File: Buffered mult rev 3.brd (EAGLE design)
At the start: 100.3 x 17.1 mm, 28 parts, among them IC1 OPA4171, IC2 OPA2171, J1 EURO_POWER_HEADERFAT_PADS

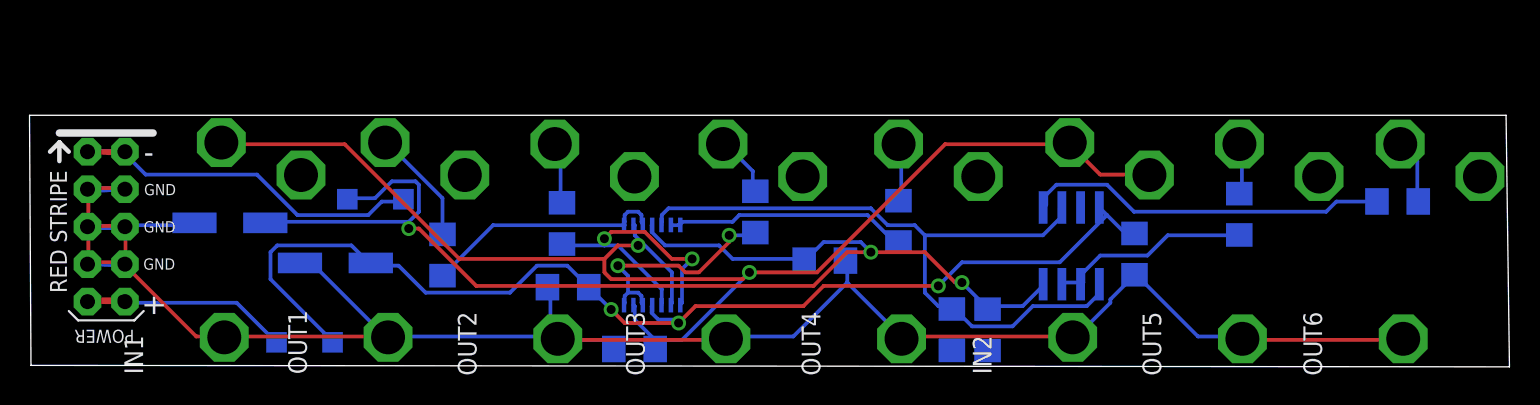
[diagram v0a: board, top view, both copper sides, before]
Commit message: minor changes
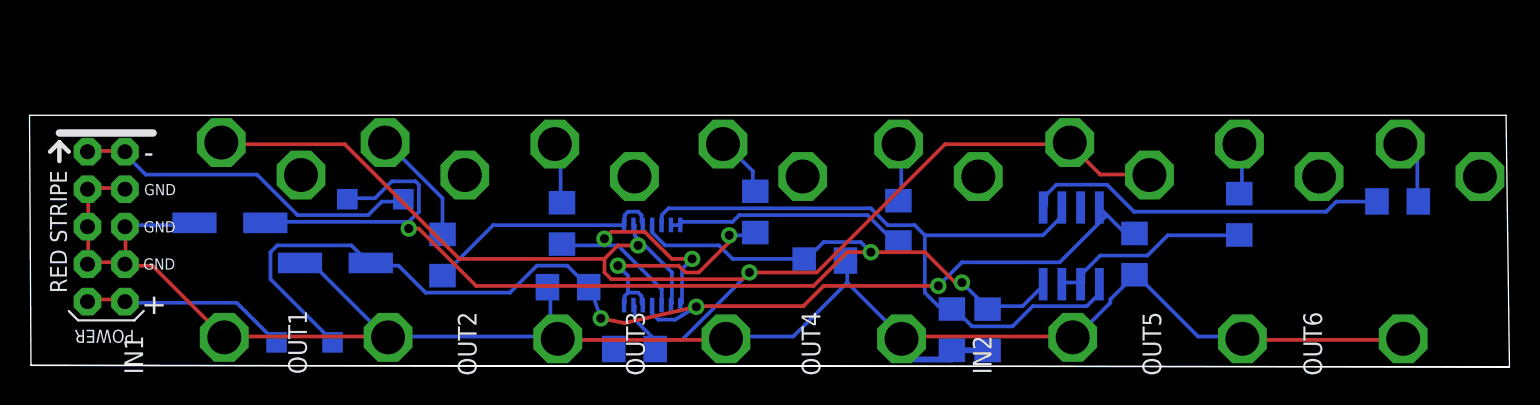
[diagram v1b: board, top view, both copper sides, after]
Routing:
- net GND: track 158.0 -> 140.2 mm, vias 11 -> 1
- net N$15: track 30.7 -> 23.8 mm, vias 3 -> 0
- net N$14: track 21.0 -> 14.1 mm, vias 3 -> 0
- net VEE: track 77.3 -> 78.9 mm
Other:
- board text added: "༼ ͒ ̶ ͒༽"
- board text added: "༼ ͒ ͓ ͒༽"
- board text added: "ヽ(°◇° )ノ"
- board text removed: "PASS DAT SHIT"

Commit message: Layout done.
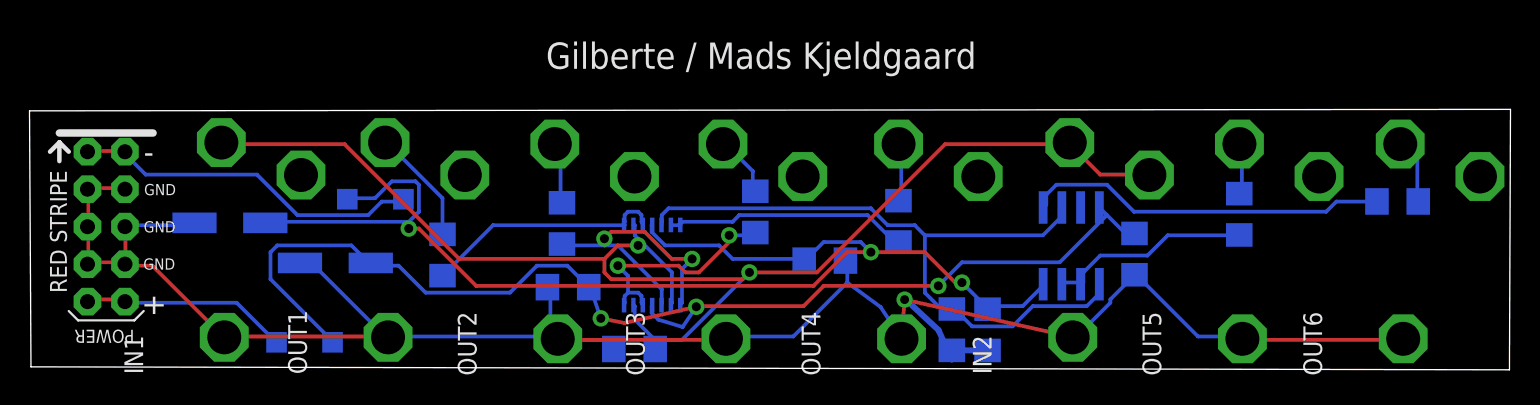
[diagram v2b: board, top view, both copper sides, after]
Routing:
- net GND: track 140.2 -> 143.3 mm
- net VEE: track 78.9 -> 79.5 mm
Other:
- board size 100.3 x 17.1 mm -> 100.4 x 17.6 mm
- board text added: "Gilberte / Mads Kjeldgaard"
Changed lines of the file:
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@@
 <board>
 <plain>
-<wire x1="100.2" y1="0" x2="99.97" y2="17.05" width="0" layer="20"/>
-<wire x1="99.97" y1="17.05" x2="-0.1" y2="17.05" width="0" layer="20"/>
-<wire x1="-0.1" y1="17.05" x2="0" y2="0.1" width="0" layer="20"/>
-<wire x1="0" y1="0.1" x2="100.2" y2="0" width="0" layer="20"/>
+<wire x1="100.2" y1="-0.2" x2="100.27" y2="17.45" width="0" layer="20"/>
+<wire x1="100.27" y1="17.45" x2="-0.1" y2="17.35" width="0" layer="20"/>
+<wire x1="-0.1" y1="17.35" x2="0" y2="0" width="0" layer="20"/>
 <text x="96.9" y="5.5" size="1.778" layer="26" rot="MR0">༼ ͒ ̶ ͒༽</text>
 <text x="56.7" y="0.7" size="1.778" layer="26" rot="MR0">༼ ͒ ͓ ͒༽</text>
@@
 <text x="84.3" y="5" size="1.778" layer="26" rot="MR0">༼ ͒ ̶ ͒༽</text>
 <text x="65.7" y="8" size="1.778" layer="26" rot="MR0">༼ ͒ ̶ ͒༽</text>
-<wire x1="0" y1="0.1" x2="100.2" y2="0" width="0" layer="20"/>
+<wire x1="0" y1="0" x2="100.2" y2="-0.2" width="0" layer="20"/>
 <text x="34.2" y="8.7" size="1.778" layer="26" rot="MR0">༼ ͒ ͓ ͒༽</text>
+<text x="34.9" y="20.2" size="1.778" layer="25">Gilberte / Mads Kjeldgaard</text>
 </plain>
 <attributes>
@@
 <wire x1="35.8902" y1="1.8288" x2="35.7" y2="1.9" width="0.254" layer="16"/>
 <wire x1="55.3212" y1="5.715" x2="55.3212" y2="7.0866" width="0.254" layer="16"/>
-<wire x1="58.9788" y1="2.0574" x2="55.3212" y2="5.715" width="0.254" layer="16"/>
+<wire x1="57.5788" y1="4.0574" x2="55.3212" y2="5.715" width="0.254" layer="16"/>
 <wire x1="55.3212" y1="7.0866" x2="55.2" y2="7.2" width="0.254" layer="16"/>
-<wire x1="58.9788" y1="2.0574" x2="59" y2="1.9" width="0.254" layer="16"/>
+<wire x1="57.5788" y1="4.0574" x2="59" y2="1.9" width="0.254" layer="16"/>
 <wire x1="51.6636" y1="2.0574" x2="47.3202" y2="2.0574" width="0.254" layer="16"/>
 <wire x1="55.3212" y1="5.715" x2="51.6636" y2="2.0574" width="0.254" layer="16"/>
@@
 <wire x1="35.8902" y1="1.8288" x2="35.7" y2="1.9" width="0.254" layer="1"/>
 <wire x1="47.0916" y1="1.8288" x2="47.1" y2="1.9" width="0.254" layer="1"/>
-<wire x1="59.2074" y1="2.0574" x2="70.4088" y2="2.0574" width="0.254" layer="1"/>
+<wire x1="59.2074" y1="4.5574" x2="70.4088" y2="2.0574" width="0.254" layer="1"/>
 <wire x1="70.4088" y1="2.0574" x2="70.6" y2="2" width="0.254" layer="1"/>
-<wire x1="59.2074" y1="2.0574" x2="59" y2="1.9" width="0.254" layer="1"/>
+<wire x1="59.2074" y1="4.5574" x2="59" y2="1.9" width="0.254" layer="1"/>
 <wire x1="34.7472" y1="2.0574" x2="24.2316" y2="2.0574" width="0.254" layer="16"/>
 <wire x1="35.2044" y1="2.5146" x2="34.7472" y2="2.0574" width="0.254" layer="16"/>
@@
 <wire x1="6.4008" y1="6.858" x2="6.37" y2="6.96" width="0.254" layer="1"/>
 <wire x1="13.0302" y1="2.0574" x2="13.1" y2="2" width="0.254" layer="1"/>
-<via x="59.2074" y="2.0574" extent="1-16" drill="0.6" shape="square"/>
-<wire x1="59.2074" y1="2.0574" x2="59.1" y2="2.0574" width="0.4064" layer="16"/>
-<wire x1="59.1" y1="2.0574" x2="59.1" y2="0.5" width="0.4064" layer="16"/>
-<wire x1="59.1" y1="0.5" x2="62.41" y2="0.5" width="0.4064" layer="16"/>
+<via x="59.2074" y="4.5574" extent="1-16" drill="0.6" shape="square"/>
+<wire x1="59.2074" y1="4.5574" x2="59.2426" y2="4.6" width="0.4064" layer="16"/>
+<wire x1="59.2426" y1="4.6" x2="61.5" y2="2.5" width="0.4064" layer="16"/>
+<wire x1="61.5" y1="2.5" x2="62.41" y2="0.5" width="0.4064" layer="16"/>
 <wire x1="62.41" y1="0.5" x2="62.41" y2="1.12" width="0.4064" layer="16"/>
 <wire x1="62.41" y1="1.12" x2="64.83" y2="1.12" width="0.4064" layer="16"/>
@@
 <wire x1="42.0624" y1="3.6576" x2="42.0624" y2="4.1148" width="0.254" layer="16"/>
 <wire x1="42.5196" y1="3.2004" x2="42.0624" y2="3.6576" width="0.254" layer="16"/>
-<wire x1="43.6626" y1="3.2004" x2="42.5196" y2="3.2004" width="0.254" layer="16"/>
-<wire x1="45.0912" y1="4.0718" x2="43.6626" y2="3.2004" width="0.254" layer="16"/>
+<wire x1="44.1626" y1="2.7004" x2="42.5196" y2="3.2004" width="0.254" layer="16"/>
+<wire x1="45.0912" y1="4.0718" x2="44.1626" y2="2.7004" width="0.254" layer="16"/>
 <wire x1="40.2336" y1="2.9718" x2="45.0912" y2="4.0718" width="0.254" layer="1"/>
 <wire x1="38.6192" y1="3.2862" x2="40.2336" y2="2.9718" width="0.254" layer="1"/>
